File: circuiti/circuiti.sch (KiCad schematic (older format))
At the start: 31 parts, among them Q1 IRFZ44N, Q2 BC547B, Q3 BC547B, Q4 TIP32C, Q5 TIP31C, SW1 SW_DIP_x01

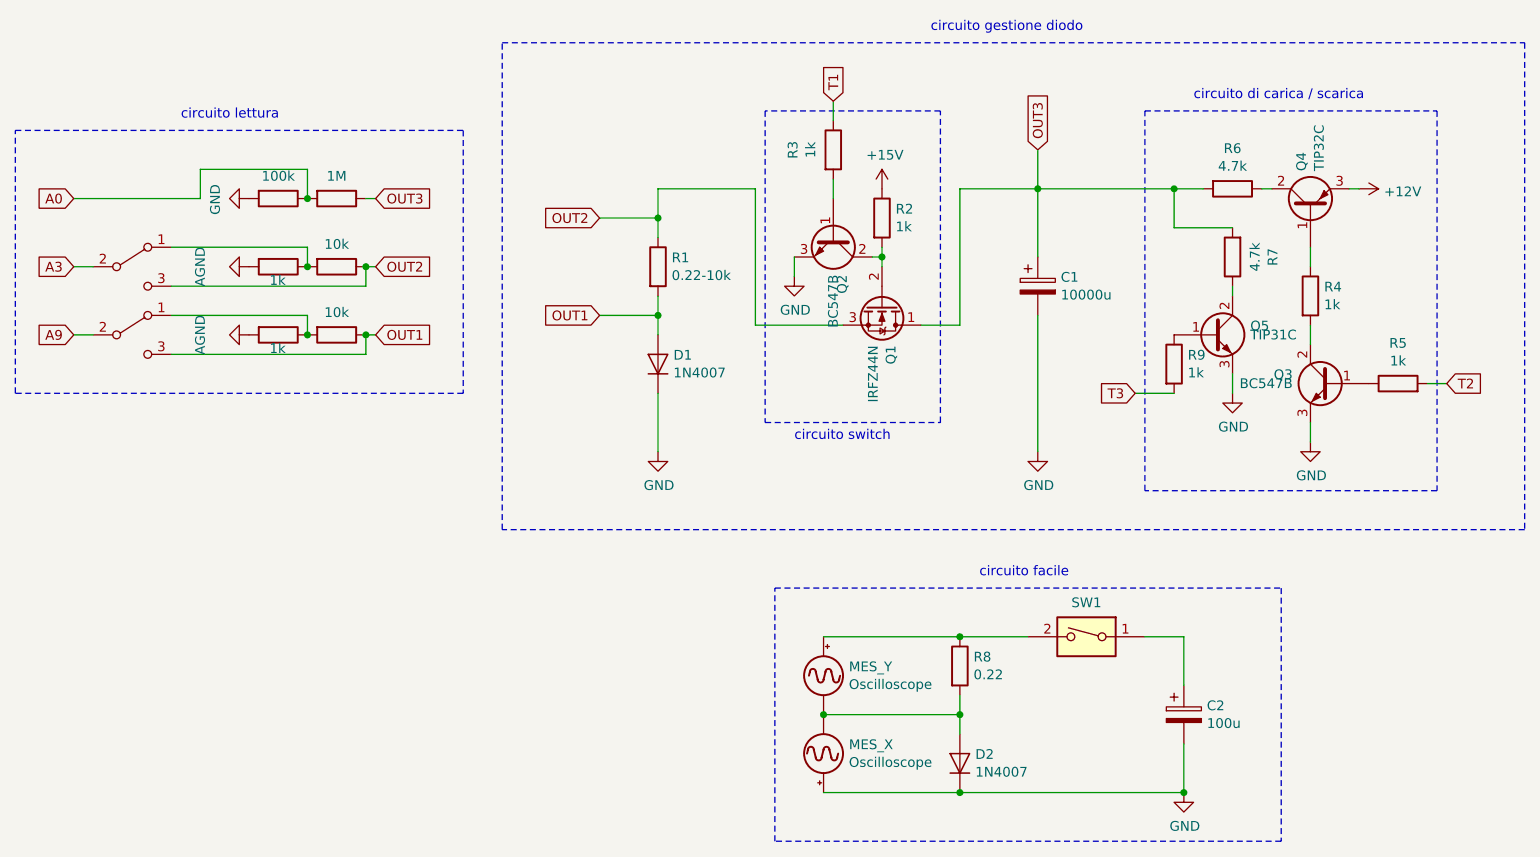
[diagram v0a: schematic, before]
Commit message: update circuito
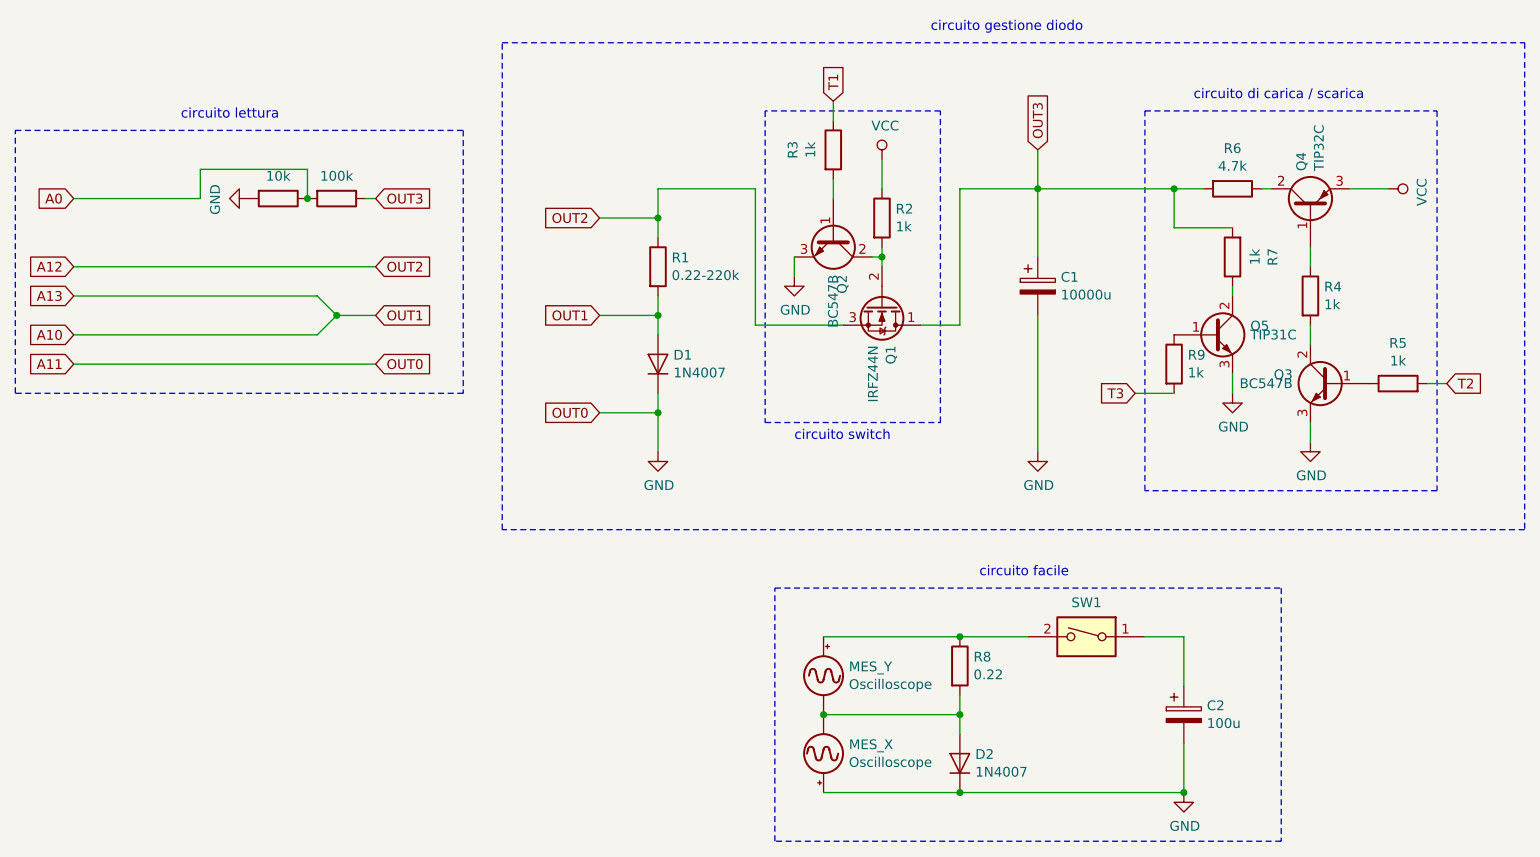
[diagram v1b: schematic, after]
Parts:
- removed AGND (x2): GND, symbol power:GND
- removed R? (x2): 10k, symbol Device:R
- removed R? (x2): 1k, symbol Device:R
- removed SW? (x2): SW_DPDT_x2, symbol Switch:SW_DPDT_x2
- R1: value 0.22-10k -> 0.22-220k
- R7: value 4.7k -> 1k
- R?: value 1M -> 100k
- R?: value 100k -> 10k
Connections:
- net +15V is gone; now on net VCC: R2.1
- net +12V renamed VCC
- net OUT1 renamed A10
- net OUT2 renamed A12
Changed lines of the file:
@@
 P 6500 1950
 F 0 "R1" H 6570 1996 50  0000 L CNN
-F 1 "0.22-10k" H 6570 1905 50  0000 L CNN
+F 1 "0.22-220k" H 6570 1905 50  0000 L CNN
 F 2 "" V 6430 1950 50  0001 C CNN
 F 3 "~" H 6500 1950 50  0001 C CNN
@@
 F 3 "~" H 7650 1700 50  0001 C CNN
 	1    7650 1700
-	1    0    0    -1
-$EndComp
-$Comp
-L power:+15V #PWR?
-U 1 1 5E317383
-P 7650 1550
-F 0 "#PWR?" H 7650 1400 50  0001 C CNN
-F 1 "+15V" H 7665 1723 50  0000 C CNN
-F 2 "" H 7650 1550 50  0001 C CNN
-F 3 "" H 7650 1550 50  0001 C CNN
-	1    7650 1550
 	1    0    0    -1
 $EndComp
@@
 Wire Wire Line
 	9850 2750 9850 2850
-$Comp
-L power:+12V #PWR?
-U 1 1 5E341474
-P 10100 1550
-F 0 "#PWR?" H 10100 1400 50  0001 C CNN
-F 1 "+12V" V 10115 1678 50  0000 L CNN
-F 2 "" H 10100 1550 50  0001 C CNN
-F 3 "" H 10100 1550 50  0001 C CNN
-	1    10100 1550
-	0    1    1    0
-$EndComp
-Wire Wire Line
-	10050 1550 10100 1550
+Wire Wire Line
+	10050 1550 10250 1550
 Text GLabel 10550 2550 2    50   Input ~ 0
 T2
@@
 $EndComp
 Wire Wire Line
-	6500 2900 6500 2600
+	6500 2900 6500 2700
 $Comp
 L Diode:1N4007 D1
@@
 Wire Wire Line
 	9450 2050 9450 2100
-Text GLabel 5050 2300 2    50   Input ~ 0
+Text GLabel 5050 2200 2    50   Input ~ 0
 OUT1
 Text GLabel 8450 1350 1    50   Input ~ 0
@@
 P 9450 1900
 F 0 "R7" V 9243 1900 50  0000 C CNN
-F 1 "4.7k" V 9334 1900 50  0000 C CNN
+F 1 "1k" V 9334 1900 50  0000 C CNN
 F 2 "" V 9380 1900 50  0001 C CNN
 F 3 "~" H 9450 1900 50  0001 C CNN
@@
 P 4550 1600
 F 0 "R?" H 4620 1646 50  0001 L CNN
-F 1 "100k" V 4435 1600 50  0000 C CNN
+F 1 "10k" V 4435 1600 50  0000 C CNN
 F 2 "" V 4480 1600 50  0001 C CNN
 F 3 "~" H 4550 1600 50  0001 C CNN
@@
 Text GLabel 3500 1600 0    50   Input ~ 0
 A0
-$Comp
-L Switch:SW_DPDT_x2 SW?
-U 1 1 5E3D2DC7
-P 3800 2300
-F 0 "SW?" H 3800 2585 50  0001 C CNN
-F 1 "SW_DPDT_x2" H 3800 2494 50  0001 C CNN
-F 2 "" H 3800 2300 50  0001 C CNN
-F 3 "~" H 3800 2300 50  0001 C CNN
-	1    3800 2300
-	1    0    0    -1
-$EndComp
-Wire Wire Line
-	5000 2300 5050 2300
-$Comp
-L Device:R R?
-U 1 1 5E3416D5
-P 4850 2300
-F 0 "R?" H 4920 2346 50  0001 L CNN
-F 1 "10k" V 4735 2300 50  0000 C CNN
-F 2 "" V 4780 2300 50  0001 C CNN
-F 3 "~" H 4850 2300 50  0001 C CNN
-	1    4850 2300
-	0    1    1    0
-$EndComp
-$Comp
-L power:GND AGND
-U 1 1 5E3416E1
-P 4400 2300
-F 0 "AGND" H 4400 2050 50  0000 C CNN
-F 1 "GND" H 4405 2127 50  0001 C CNN
-F 2 "" H 4400 2300 50  0001 C CNN
-F 3 "" H 4400 2300 50  0001 C CNN
-	1    4400 2300
-	0    1    1    0
-$EndComp
-Wire Wire Line
-	4000 2200 4700 2200
-Wire Wire Line
-	4700 2200 4700 2300
-Connection ~ 4700 2300
-Wire Wire Line
-	5000 2400 5000 2300
-Connection ~ 5000 2300
-$Comp
-L Device:R R?
-U 1 1 5E3416DB
-P 4550 2300
-F 0 "R?" H 4620 2346 50  0001 L CNN
-F 1 "1k" V 4620 2255 50  0000 L CNN
-F 2 "" V 4480 2300 50  0001 C CNN
-F 3 "~" H 4550 2300 50  0001 C CNN
-	1    4550 2300
-	0    1    1    0
-$EndComp
-Wire Wire Line
-	4000 2400 5000 2400
 Text GLabel 5050 1950 2    50   Input ~ 0
 OUT2
-$Comp
-L Switch:SW_DPDT_x2 SW?
-U 1 1 5E34A161
-P 3800 1950
-F 0 "SW?" H 3800 2235 50  0001 C CNN
-F 1 "SW_DPDT_x2" H 3800 2144 50  0001 C CNN
-F 2 "" H 3800 1950 50  0001 C CNN
-F 3 "~" H 3800 1950 50  0001 C CNN
-	1    3800 1950
-	1    0    0    -1
-$EndComp
-Wire Wire Line
-	5000 1950 5050 1950
-$Comp
-L Device:R R?
-U 1 1 5E34A168
-P 4850 1950
-F 0 "R?" H 4920 1996 50  0001 L CNN
-F 1 "10k" V 4735 1950 50  0000 C CNN
-F 2 "" V 4780 1950 50  0001 C CNN
-F 3 "~" H 4850 1950 50  0001 C CNN
-	1    4850 1950
-	0    1    1    0
-$EndComp
-Wire Wire Line
-	4000 1850 4700 1850
-Wire Wire Line
-	4700 1850 4700 1950
-Connection ~ 4700 1950
-Wire Wire Line
-	5000 2050 5000 1950
-Connection ~ 5000 1950
-$Comp
-L Device:R R?
-U 1 1 5E34A179
-P 4550 1950
-F 0 "R?" H 4620 1996 50  0001 L CNN
-F 1 "1k" V 4620 1905 50  0000 L CNN
-F 2 "" V 4480 1950 50  0001 C CNN
-F 3 "~" H 4550 1950 50  0001 C CNN
-	1    4550 1950
-	0    1    1    0
-$EndComp
-Wire Wire Line
-	4000 2050 5000 2050
 $Comp
 L Device:R R?
@@
 P 4850 1600
 F 0 "R?" H 4920 1646 50  0001 L CNN
-F 1 "1M" V 4735 1600 50  0000 C CNN
+F 1 "100k" V 4735 1600 50  0000 C CNN
 F 2 "" V 4780 1600 50  0001 C CNN
 F 3 "~" H 4850 1600 50  0001 C CNN
@@
 Connection ~ 4700 1600
 Text GLabel 3500 1950 0    50   Input ~ 0
-A3
+A12
 Text GLabel 3500 2300 0    50   Input ~ 0
-A9
-Wire Wire Line
-	3500 1950 3600 1950
-Wire Wire Line
-	3600 2300 3500 2300
+A10
 Wire Notes Line
 	3200 1250 5500 1250
@@
 	1    0    0    -1
 $EndComp
-$Comp
-L power:GND AGND
-U 1 1 5E37666D
-P 4400 1950
-F 0 "AGND" H 4400 1700 50  0000 C CNN
-F 1 "GND" H 4405 1777 50  0001 C CNN
-F 2 "" H 4400 1950 50  0001 C CNN
-F 3 "" H 4400 1950 50  0001 C CNN
-	1    4400 1950
-	0    1    1    0
-$EndComp
+Text GLabel 6200 2700 0    50   Input ~ 0
+OUT0
+Wire Wire Line
+	6200 2700 6500 2700
+Connection ~ 6500 2700
+Wire Wire Line
+	6500 2700 6500 2600
+Text GLabel 3500 2100 0    50   Input ~ 0
+A13
+Text GLabel 3500 2450 0    50   Input ~ 0
+A11
+Text GLabel 5050 2450 2    50   Input ~ 0
+OUT0
+Wire Wire Line
+	3500 1950 5050 1950
+Wire Wire Line
+	3500 2450 5050 2450
+Wire Wire Line
+	3500 2300 4750 2300
+Wire Wire Line
+	4750 2300 4850 2200
+Wire Wire Line
+	4850 2200 5050 2200
+Connection ~ 4850 2200
+Wire Wire Line
+	3500 2100 4750 2100
+Wire Wire Line
+	4750 2100 4850 2200
+$Comp
+L power:VCC #PWR?
+U 1 1 5E577E93
+P 10250 1550
+F 0 "#PWR?" H 10250 1400 50  0001 C CNN
+F 1 "VCC" H 10267 1723 50  0000 C CNN
+F 2 "" H 10250 1550 50  0001 C CNN
+F 3 "" H 10250 1550 50  0001 C CNN
+	1    10250 1550
+	0    1    1    0
+$EndComp
+$Comp
+L power:VCC #PWR?
+U 1 1 5E57EFD6
+P 7650 1400
+F 0 "#PWR?" H 7650 1250 50  0001 C CNN
+F 1 "VCC" H 7667 1573 50  0000 C CNN
+F 2 "" H 7650 1400 50  0001 C CNN
+F 3 "" H 7650 1400 50  0001 C CNN
+	1    7650 1400
+	1    0    0    -1
+$EndComp
+Wire Wire Line
+	7650 1400 7650 1550
 $EndSCHEMATC
